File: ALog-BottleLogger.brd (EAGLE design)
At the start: 120.7 x 44.5 mm, 98 parts, among them IC2 ATMEGA644M, J6 5.5x2.1mm Barrel, Q1 220mA/50V/3.5Ω, Q4 4.3A/20V/54mΩ, Q5 4.3A/20V/54mΩ, Q6 4.3A/20V/54mΩ, Q7 4.3A/20V/54mΩ, Q8 220mA/50V/3.5Ω, Q9 220mA/50V/3.5Ω, U2 FT231X-Q

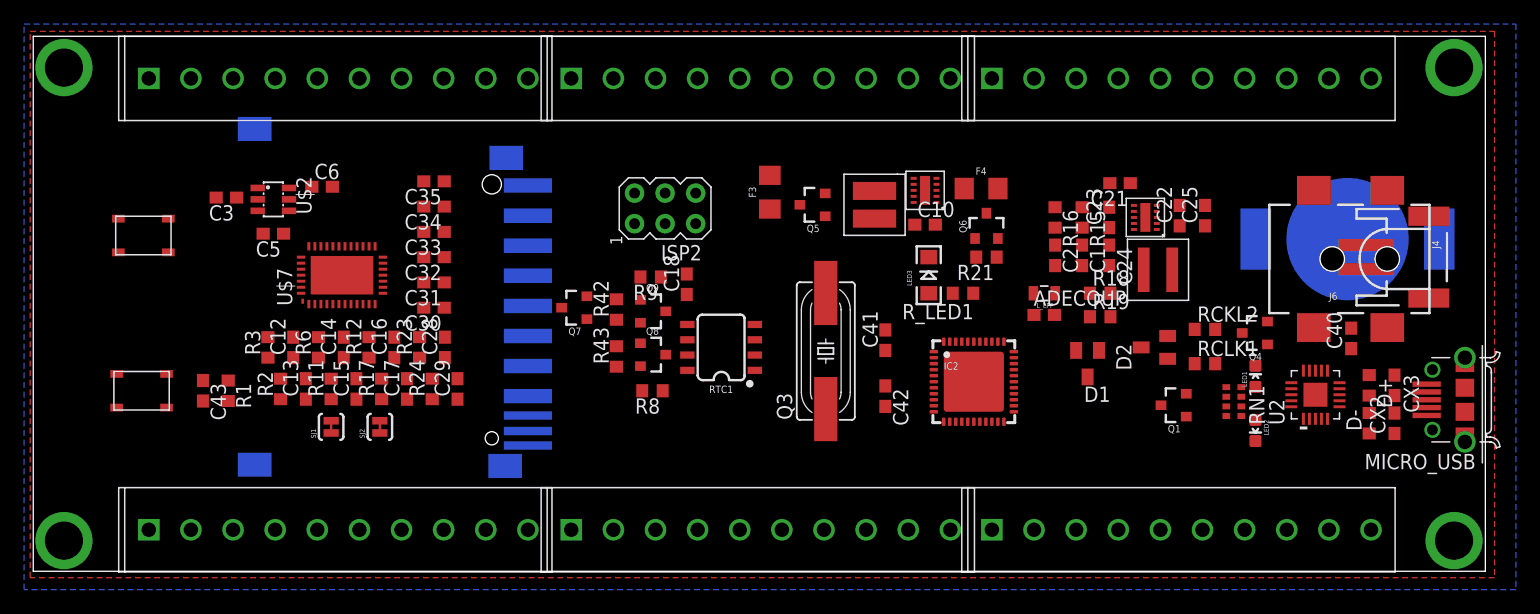
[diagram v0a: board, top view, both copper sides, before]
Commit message: fully routed, looking for review
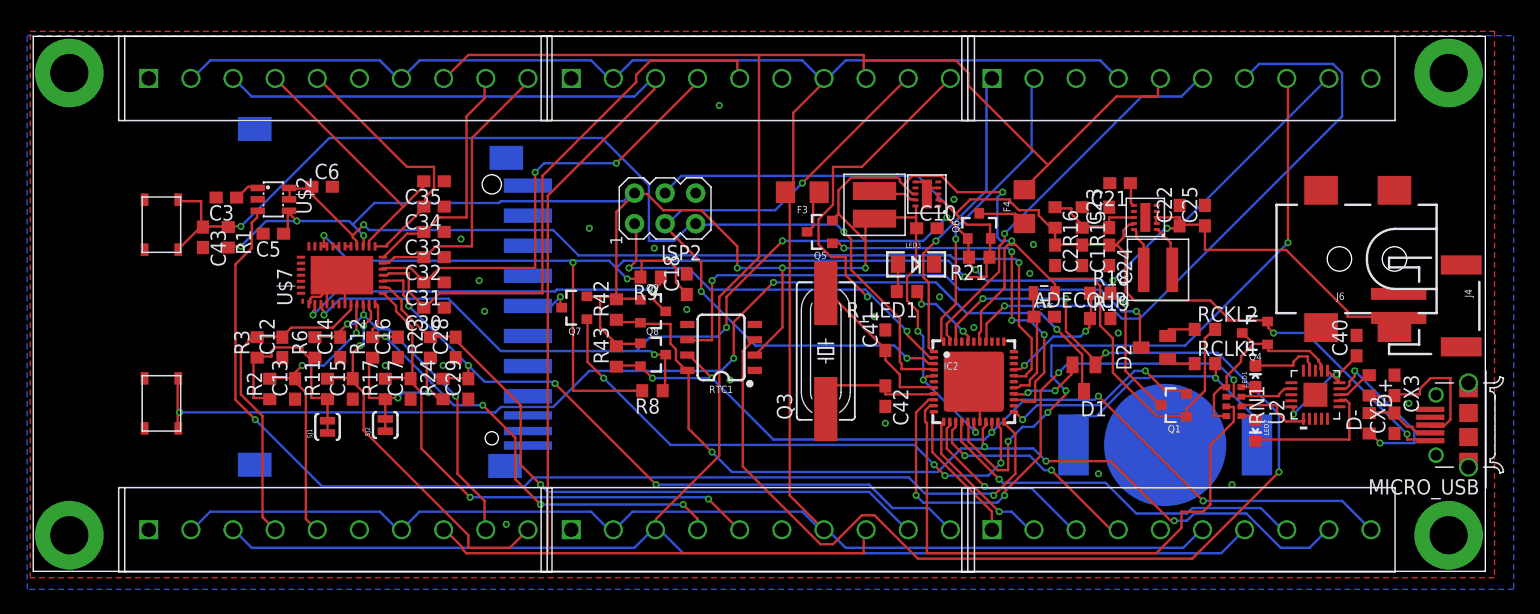
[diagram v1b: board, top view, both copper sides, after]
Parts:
- moved CLOCK_BATT 22.8 mm to (94.0, 10.5), turned to 180 degrees
- moved S1 14.0 mm to (10.7, 13.9), turned to 270 degrees
- moved U$4 13.9 mm to (10.7, 28.8), turned to 90 degrees
- moved C43 12.8 mm to (14.1, 27.8)
- moved R1 12.8 mm to (16.2, 27.8)
- moved J4 4.87 mm to (117.2, 22.1)
- moved R_LED1 4.65 mm to (72.6, 23.2)
- moved F4 3.90 mm to (82.3, 30.3), turned to 90 degrees
- moved F3 2.70 mm to (63.9, 31.5), turned to 180 degrees
- moved Q5 2.33 mm to (65.4, 28.2)
- moved MICRO_USB 2.12 mm to (119.2, 12.2)
- moved LED3 1.38 mm to (73.3, 25.5), turned to 0 degrees
- moved D1 1.24 mm to (87.3, 16.1)
- moved C12 0.90 mm to (20.7, 18.6)
- moved R2 0.90 mm to (19.6, 15.2)
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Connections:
- net +3V3: no longer J14.P$2
- net 1.8V_REF: no longer J14.P$1
- net ADC10: now also J14.P$10; no longer J15.P$2
- net ADC11: now also J14.P$9; no longer J15.P$1
- net ADC12: now also J14.P$5; no longer J14.P$7
- net ADC13: now also J14.P$4; no longer J14.P$6
- net ADC8: now also J15.P$5; no longer J15.P$7
- net ADC9: now also J15.P$4; no longer J15.P$6
- net BATT+: now also J2.P$9
- net D15~: now also J2.P$8; no longer J2.P$10
- net D3~: now also J2.P$6; no longer J2.P$8
- net EXT_3.3V: now also J14.P$2, J14.P$7, J15.P$2, J15.P$7, J2.P$4; no longer J14.P$4, J14.P$9, J15.P$4, J15.P$9, J2.P$6
- net EXT_5V: now also J14.P$8, J15.P$8, J2.P$5; no longer J14.P$10, J15.P$10, J2.P$7
- net EXT_5V1: now also J14.P$3, J15.P$3; no longer J14.P$5, J15.P$5
- net GND: now also J14.P$1, J14.P$6, J15.P$1, J15.P$6, J2.P$10, J2.P$3; no longer J14.P$3, J14.P$8, J15.P$3, J15.P$8, J2.P$5
- net MCU_ADC0: now also J2.P$7; no longer J2.P$9
- net MISO/D6: now also J15.P$10; no longer J2.P$2
- net MOSI/D5: now also J2.P$1; no longer J2.P$3
- net SCK/D7: now also J15.P$9; no longer J2.P$1
- net SS/D4: now also J2.P$2; no longer J2.P$4
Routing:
- net EXT_3.3V: track 0.00 -> 211.8 mm
- net EXT_5V: track 0.00 -> 203.2 mm
- net +3V3: track 0.00 -> 195.7 mm, vias 0 -> 11
- net +5V: track 0.00 -> 149.8 mm, vias 0 -> 6
- net EXT_5V1: track 0.00 -> 117.4 mm
- net RTC_INT: track 0.00 -> 104.2 mm, vias 0 -> 4
- net SDA_HV: track 0.00 -> 95.7 mm, vias 0 -> 7
- net N$39: track 0.00 -> 91.1 mm, vias 0 -> 4
- net 1.8V_EN: track 0.00 -> 90.6 mm, vias 0 -> 2
- net RST: track 0.00 -> 86.9 mm, vias 0 -> 2
- net 1.8V_REF: track 0.00 -> 77.7 mm, vias 0 -> 2
- net SCL: track 0.00 -> 76.7 mm, vias 0 -> 4
- net SDA: track 0.00 -> 75.2 mm, vias 0 -> 5
- net ADC7: track 0.00 -> 60.0 mm, vias 0 -> 4
- net MISO/D6: track 0.00 -> 59.5 mm, vias 0 -> 3
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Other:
- board text added: "BATT"
- board text removed: "1.8V_REF"
- board text removed: "3V3_REF"
